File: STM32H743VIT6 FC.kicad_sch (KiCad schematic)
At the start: 79 parts, among them SW2 SW_Push, U1 TPS54302DDCR, U2 USBLC6-2SC6, U3 TPS54302DDCR

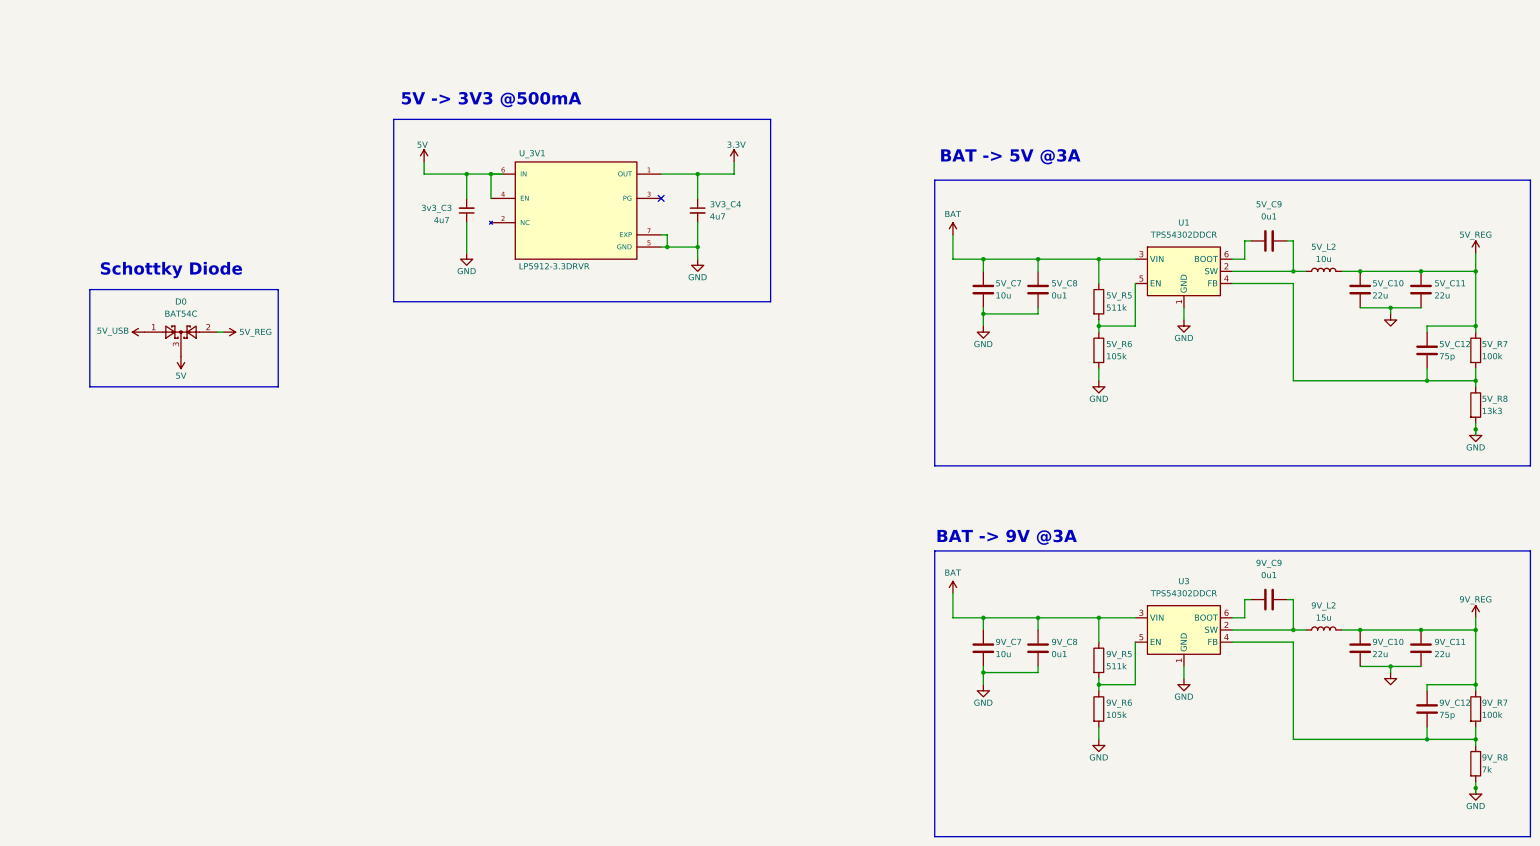
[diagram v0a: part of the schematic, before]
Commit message: nez
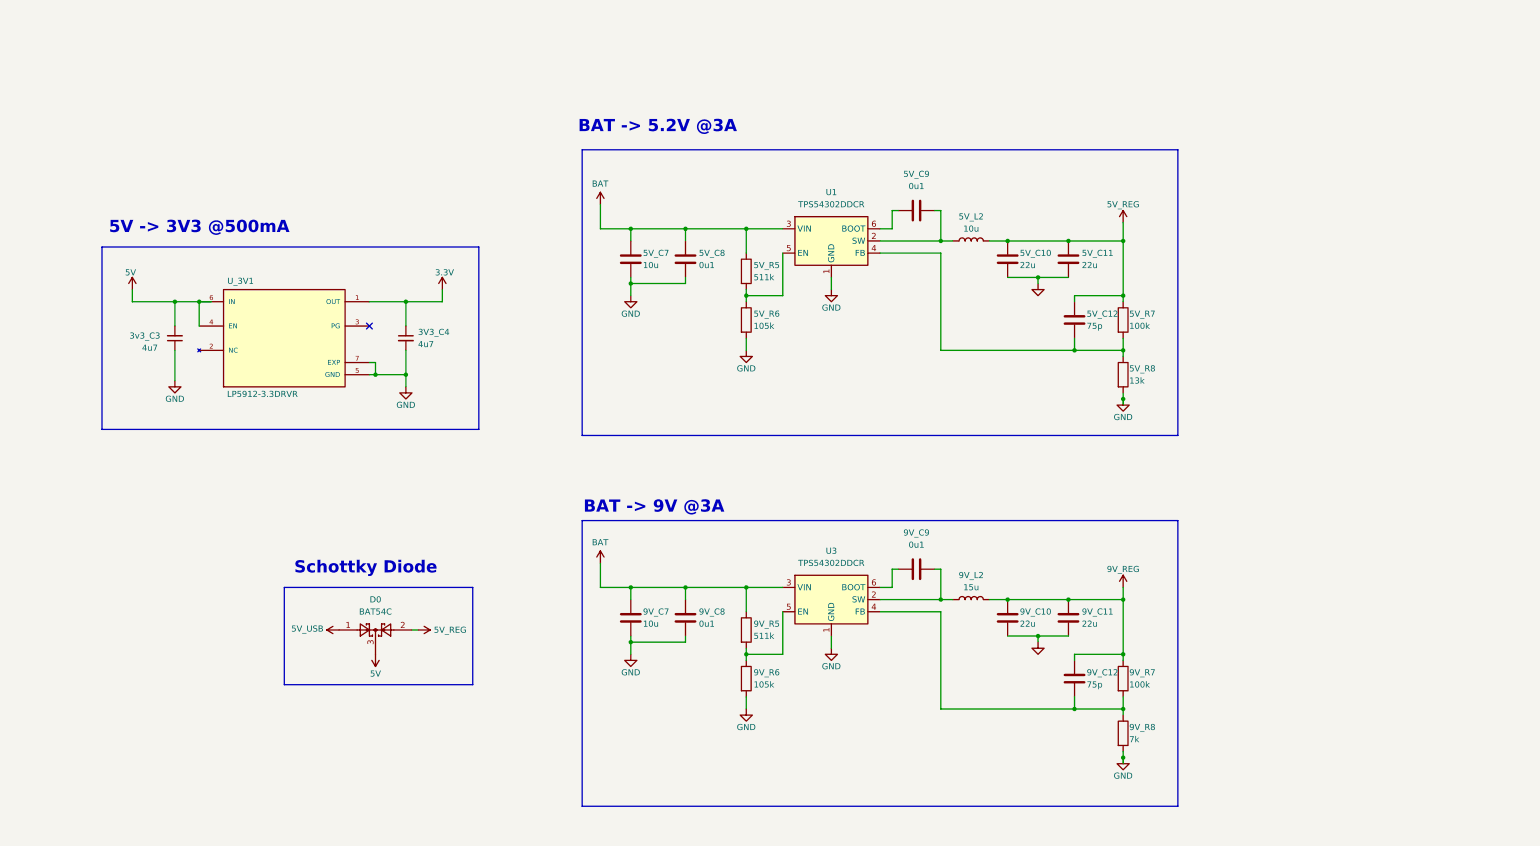
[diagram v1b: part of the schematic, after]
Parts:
- 5V_R8: value 13k3 -> 13k
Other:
- note added: "BAT -> 5.2V @3A"
- note removed: "BAT -> 5V @3A"
- moved on the sheet: 3V3_C4, 3v3_C3, 5V_C10, 5V_C11, 5V_C12, 5V_C7, 5V_C8, 5V_C9, 5V_L2, 5V_R5, 5V_R6, 5V_R7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
